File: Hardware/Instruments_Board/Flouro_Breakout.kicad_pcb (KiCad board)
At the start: 2 copper layers, 12 parts, among them J1 RJ45_LED_Shielded, U1 Teensy4.1_DEV-16771, U2 3V3 OKI

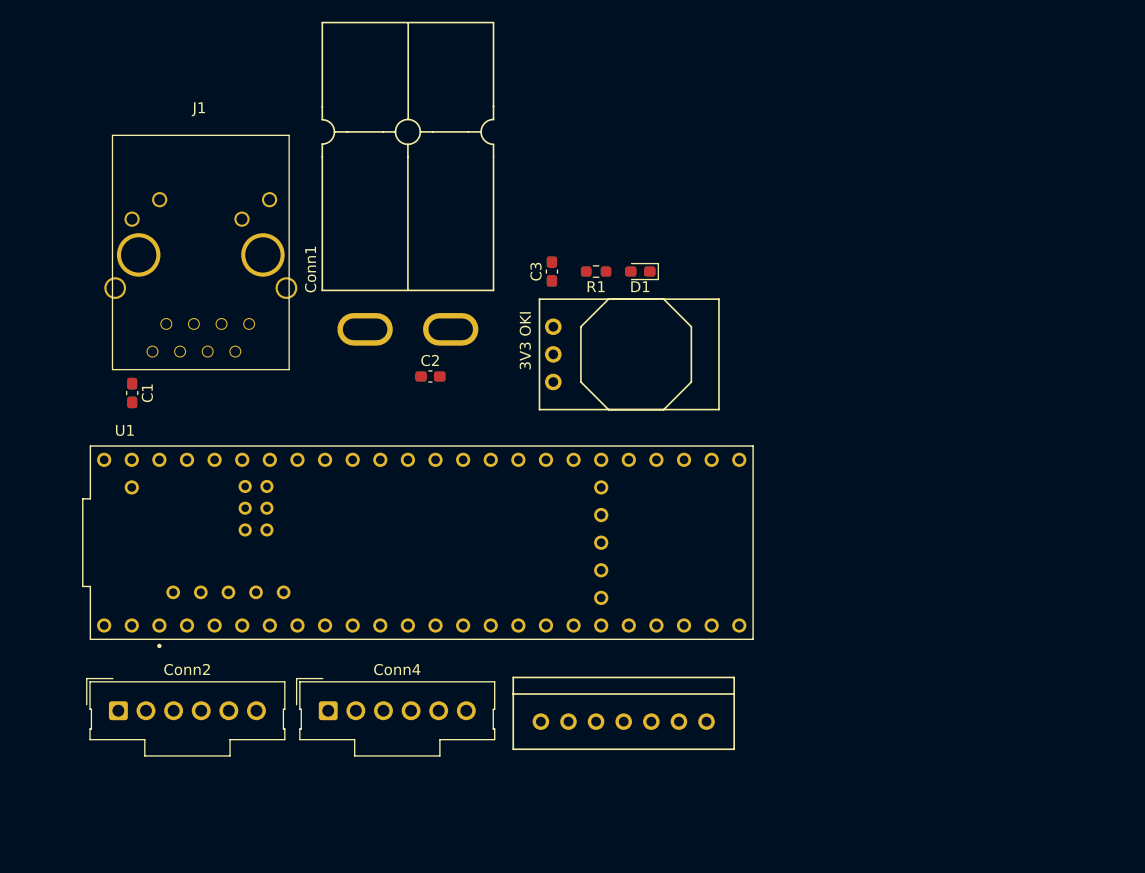
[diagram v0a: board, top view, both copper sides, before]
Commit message: Running traces
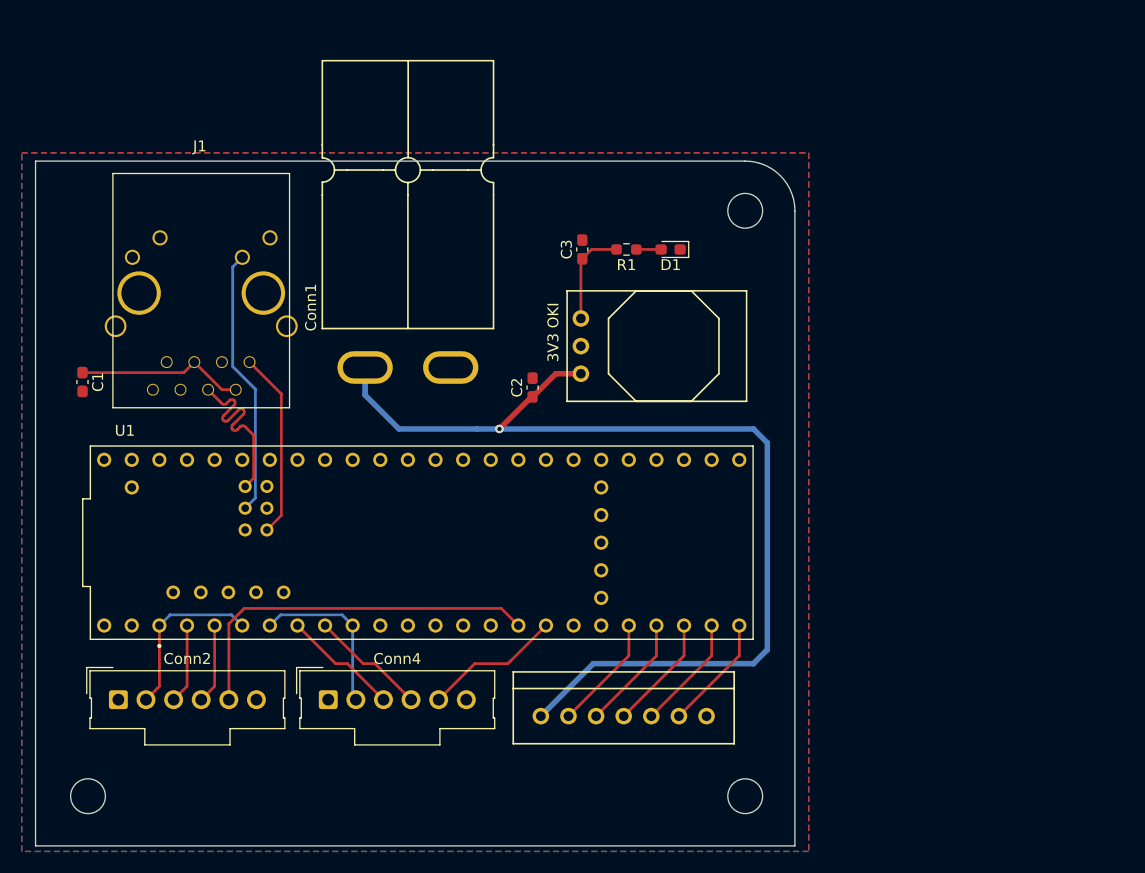
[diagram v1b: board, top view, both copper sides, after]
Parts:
- added H1: MountingHole, MountingHole:MountingHole_3.2mm_M3, F.Cu at (173.2, 52.3)
- added H2: MountingHole, MountingHole:MountingHole_3.2mm_M3, F.Cu at (173.2, 106.2)
- added H3: MountingHole, MountingHole:MountingHole_3.2mm_M3, F.Cu at (112.8, 106.2)
- R1: value 130 -> 100
- moved C2 9.45 mm to (153.7, 68.6), turned to 90 degrees
- moved C1 4.68 mm to (112.3, 68.1)
- moved J1 3.51 mm to (123.1, 46.9)
- moved Conn1 3.51 mm to (146.7, 67.1)
- moved D1 3.45 mm to (166.4, 55.9)
- moved R1 3.45 mm to (162.3, 55.9)
- moved C3 3.45 mm to (158.2, 55.9)
- moved U2 2.65 mm to (158.1, 67.3)
- moved Conn2 1.02 mm to (115.6, 97.3)
- moved Conn4 1.02 mm to (134.9, 97.3)
- moved Conn3 0.51 mm to (154.4, 98.8)
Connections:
- net Net-(J1-Pad1) renamed T+
- net Net-(J1-Pad10) renamed ETH_LED
- net Net-(J1-Pad3) renamed T-
- net Net-(J1-Pad4) renamed R+
- net Net-(J1-Pad6) renamed R-
- Conn3 pad 2: /365nm -> 365_CTRL
- Conn3 pad 3: /310nm -> 310_CTRL
- Conn3 pad 4: /280nm -> 280_CTRL
- Conn3 pad 5: /275nm -> 275_CTRL
- Conn3 pad 6: /260nm -> 260_CTRL
- U1 pad 27: /260nm -> unconnected-(U1-Pad27)
- U1 pad 28: unconnected-(U1-Pad28) -> 365_CTRL
- U1 pad 29: unconnected-(U1-Pad29) -> 310_CTRL
- U1 pad 30: unconnected-(U1-Pad30) -> 280_CTRL
- U1 pad 31: unconnected-(U1-Pad31) -> 275_CTRL
- U1 pad 32: unconnected-(U1-Pad32) -> 260_CTRL
- U1 pad 38: /275nm -> unconnected-(U1-Pad38)
- U1 pad 39: /280nm -> unconnected-(U1-Pad39)
- U1 pad 40: /310nm -> unconnected-(U1-Pad40)
- U1 pad 41: /365nm -> unconnected-(U1-Pad41)
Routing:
- net +12V: track 0.00 -> 93.4 mm, vias 0 -> 1
- net CCD_OS: track 0.00 -> 34.8 mm
- net ETH_LED: track 0.00 -> 24.7 mm
- net R+: track 0.00 -> 17.6 mm
- net T+: track 0.00 -> 17.2 mm
- net CCD_MC: track 0.00 -> 15.8 mm
- net Net-(C1-Pad1): track 0.00 -> 15.5 mm
- net CCD_MC_1: track 0.00 -> 15.4 mm
- net CCD_OS_1: track 0.00 -> 12.7 mm
- net CCD_ICG_1: track 0.00 -> 10.7 mm
- net  CCD_SH_1: track 0.00 -> 10.7 mm
- net 310_CTRL: track 0.00 -> 10.6 mm
- net 280_CTRL: track 0.00 -> 10.6 mm
- net 365_CTRL: track 0.00 -> 10.6 mm
- net 275_CTRL: track 0.00 -> 10.6 mm
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- added copper zone on B.Cu, net GND
- added copper zone on F.Cu, net GND
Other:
- board outline added: 69.9 x 63 mm

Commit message: finished fluoro breakout
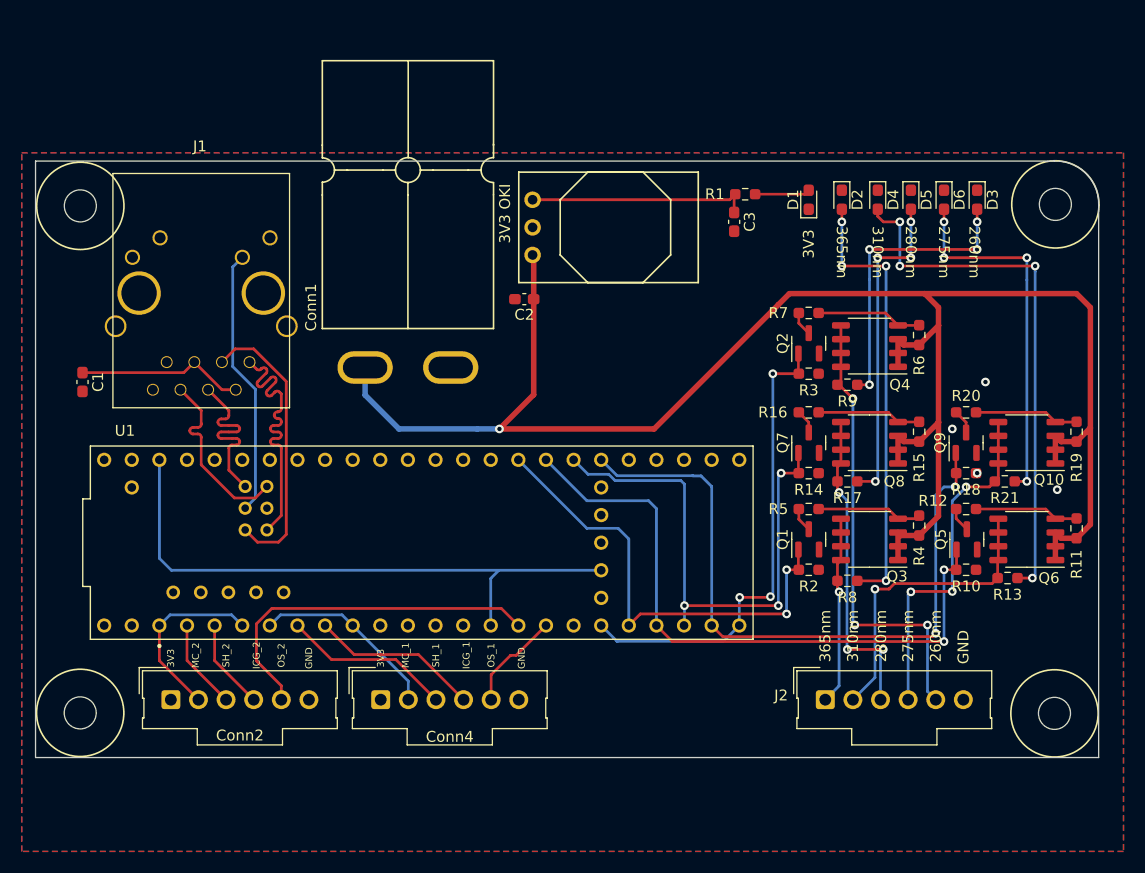
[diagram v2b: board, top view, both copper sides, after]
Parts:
- removed Conn3: Molex_SL_07, MRDT_Connectors:MOLEX_SL_07_Vertical
- added D2: Green, LED_SMD:LED_0603_1608Metric_Pad1.05x0.95mm_HandSolder, F.Cu at (182.1, 51.3)
- added D3: Green, LED_SMD:LED_0603_1608Metric_Pad1.05x0.95mm_HandSolder, F.Cu at (194.6, 51.3)
- added D4: Green, LED_SMD:LED_0603_1608Metric_Pad1.05x0.95mm_HandSolder, F.Cu at (185.4, 51.3)
- added D5: Green, LED_SMD:LED_0603_1608Metric_Pad1.05x0.95mm_HandSolder, F.Cu at (188.5, 51.3)
- added D6: Green, LED_SMD:LED_0603_1608Metric_Pad1.05x0.95mm_HandSolder, F.Cu at (191.5, 51.3)
- added H4: MountingHole, MRDT_Drill_Holes:4_40_Hole_Corner, F.Cu at (116.1, 55.9)
- added J2: Conn_01x06_Female, Connector_Molex:Molex_SL_171971-0006_1x06_P2.54mm_Vertical, F.Cu at (180.6, 97.3)
- added Q1: BSS138, Package_TO_SOT_SMD:SOT-23, F.Cu at (179.1, 82.5)
- added Q10: IRF7606PBF, Package_SO:SOP-8_3.9x4.9mm_P1.27mm, F.Cu at (199.1, 73.7)
- added Q2: BSS138, Package_TO_SOT_SMD:SOT-23, F.Cu at (179.1, 64.5)
- added Q3: IRF7606PBF, Package_SO:SOP-8_3.9x4.9mm_P1.27mm, F.Cu at (184.7, 82.5)
- added Q4: IRF7606PBF, Package_SO:SOP-8_3.9x4.9mm_P1.27mm, F.Cu at (184.7, 64.8)
- added Q5: BSS138, Package_TO_SOT_SMD:SOT-23, F.Cu at (193.6, 82.5)
- added Q6: IRF7606PBF, Package_SO:SOP-8_3.9x4.9mm_P1.27mm, F.Cu at (199.1, 82.5)
- added Q7: BSS138, Package_TO_SOT_SMD:SOT-23, F.Cu at (179.1, 73.7)
- added Q8: IRF7606PBF, Package_SO:SOP-8_3.9x4.9mm_P1.27mm, F.Cu at (184.7, 73.7)
- added Q9: BSS138, Package_TO_SOT_SMD:SOT-23, F.Cu at (193.5, 73.7)
- added R10: 4.7k, Resistor_SMD:R_0603_1608Metric_Pad0.98x0.95mm_HandSolder, F.Cu at (193.5, 85.3)
- added R11: 10k, Resistor_SMD:R_0603_1608Metric_Pad0.98x0.95mm_HandSolder, F.Cu at (203.7, 81.5)
- added R12: 10k, Resistor_SMD:R_0603_1608Metric_Pad0.98x0.95mm_HandSolder, F.Cu at (193.5, 79.8)
- added R13: 1k, Resistor_SMD:R_0603_1608Metric_Pad0.98x0.95mm_HandSolder, F.Cu at (197.4, 86.1)
- added R14: 4.7k, Resistor_SMD:R_0603_1608Metric_Pad0.98x0.95mm_HandSolder, F.Cu at (179.1, 76.5)
- added R15: 10k, Resistor_SMD:R_0603_1608Metric_Pad0.98x0.95mm_HandSolder, F.Cu at (189.2, 72.6)
- added R16: 10k, Resistor_SMD:R_0603_1608Metric_Pad0.98x0.95mm_HandSolder, F.Cu at (179.1, 70.9)
- added R17: 1k, Resistor_SMD:R_0603_1608Metric_Pad0.98x0.95mm_HandSolder, F.Cu at (182.6, 77.2)
- added R18: 4.7k, Resistor_SMD:R_0603_1608Metric_Pad0.98x0.95mm_HandSolder, F.Cu at (193.5, 76.5)
- added R19: 10k, Resistor_SMD:R_0603_1608Metric_Pad0.98x0.95mm_HandSolder, F.Cu at (203.7, 72.6)
- added R2: 4.7k, Resistor_SMD:R_0603_1608Metric_Pad0.98x0.95mm_HandSolder, F.Cu at (179.1, 85.3)
- added R20: 10k, Resistor_SMD:R_0603_1608Metric_Pad0.98x0.95mm_HandSolder, F.Cu at (193.5, 70.9)
- added R21: 1k, Resistor_SMD:R_0603_1608Metric_Pad0.98x0.95mm_HandSolder, F.Cu at (197.1, 77.2)
- added R3: 4.7k, Resistor_SMD:R_0603_1608Metric_Pad0.98x0.95mm_HandSolder, F.Cu at (179.1, 67.3)
- added R4: 10k, Resistor_SMD:R_0603_1608Metric_Pad0.98x0.95mm_HandSolder, F.Cu at (189.2, 81.3)
- added R5: 10k, Resistor_SMD:R_0603_1608Metric_Pad0.98x0.95mm_HandSolder, F.Cu at (179.1, 79.8)
- added R6: 10k, Resistor_SMD:R_0603_1608Metric_Pad0.98x0.95mm_HandSolder, F.Cu at (189.2, 63.8)
- added R7: 10k, Resistor_SMD:R_0603_1608Metric_Pad0.98x0.95mm_HandSolder, F.Cu at (179.1, 61.7)
- added R8: 1k, Resistor_SMD:R_0603_1608Metric_Pad0.98x0.95mm_HandSolder, F.Cu at (182.6, 86.4)
- added R9: 1k, Resistor_SMD:R_0603_1608Metric_Pad0.98x0.95mm_HandSolder, F.Cu at (182.6, 68.3)
- H1, H2, H3: footprint MountingHole:MountingHole_3.2mm_M3 -> MRDT_Drill_Holes:4_40_Hole_Corner
- moved H2 27.1 mm to (197.7, 94.5), turned to -90 degrees
- moved H1 24.8 mm to (197.8, 55.7)
- moved C3 14.2 mm to (172.2, 53.3), turned to -90 degrees
- moved D1 13.5 mm to (179.1, 51.3), turned to 90 degrees
- moved H3 12.1 mm to (116.1, 94.5), turned to 180 degrees
- moved R1 12.0 mm to (173.2, 50.8)
- moved U2 11.8 mm to (153.7, 56.4)
- moved C2 8.16 mm to (152.9, 60.5), turned to 180 degrees
- moved Conn2 4.83 mm to (120.4, 97.3)
- moved Conn4 4.83 mm to (139.7, 97.3)
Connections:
- U1 pad 27: unconnected-(U1-Pad27) -> 260_CTRL
- U1 pad 38: unconnected-(U1-Pad38) -> 275_CTRL
- U1 pad 39: unconnected-(U1-Pad39) -> 280_CTRL
- U1 pad 40: unconnected-(U1-Pad40) -> 310_CTRL
- U1 pad 41: unconnected-(U1-Pad41) -> 365_CTRL
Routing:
- net +12V: track 93.4 -> 169.1 mm
- net Net-(U1-Pad3.3V_1): track 0.00 -> 55.5 mm
- net 275_CTRL: track 10.6 -> 63.1 mm, vias 0 -> 2
- net Net-(D4-Pad2): track 0.00 -> 49.6 mm, vias 0 -> 4
- net 310_CTRL: track 10.6 -> 59.4 mm, vias 0 -> 2
- net 260nm: track 0.00 -> 42.3 mm, vias 0 -> 3
- net Net-(D2-Pad2): track 0.00 -> 40.9 mm, vias 0 -> 4
- net 280_CTRL: track 10.6 -> 48.6 mm, vias 0 -> 3
- net Net-(D6-Pad2): track 0.00 -> 33.8 mm, vias 0 -> 4
- net 260_CTRL: track 10.6 -> 44.2 mm, vias 0 -> 3
- net 365_CTRL: track 10.6 -> 43.1 mm, vias 0 -> 2
- net 275nm: track 0.00 -> 32.4 mm, vias 0 -> 3
- net Net-(D5-Pad2): track 0.00 -> 29.8 mm, vias 0 -> 4
- net 280nm: track 0.00 -> 29.5 mm, vias 0 -> 3
- net 310nm: track 0.00 -> 28.4 mm, vias 0 -> 1
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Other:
- board size 69.9 x 63 mm -> 97.8 x 54.9 mm
- board text added: "260nm"
- board text added: "275nm"
- board text added: "280nm"
- board text added: "310nm"
- board text added: "365nm"
- board text added: "3V3"
- board text added: "GND"
- board text added: "ICG_1"
- board text added: "ICG_2"
- board text added: "MC_1"
- board text added: "MC_2"
- board text added: "OS_1"
- board text added: "OS_2"
- board text added: "SH_1"
- board text added: "SH_2"
